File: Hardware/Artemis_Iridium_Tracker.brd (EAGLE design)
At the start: 63.5 x 69.8 mm, 199 parts, among them J1 IRIDIUM_9603N, J2 USB-C, J6 uFL, J7 SMA-, Q1 DMG3414U-7, Q2 DMG3415U-7, Q3 DMG3415U-7, Q4 2N2222, U1 CH340E_MSOP10, U10 MCP111T-240E/TT, U2 LTC3225EDDB#TRMPBF, U3 ADM4210-1, U4 UBLOX_ZOE_M8-0-10, U5 AS179-92LF, U6 MS8607-02BA01, U7 ARTEMIS_MODULESMD, U8 AP3429A, U9 MCP73831, X1 32.768kHz, X2 32.768kHz

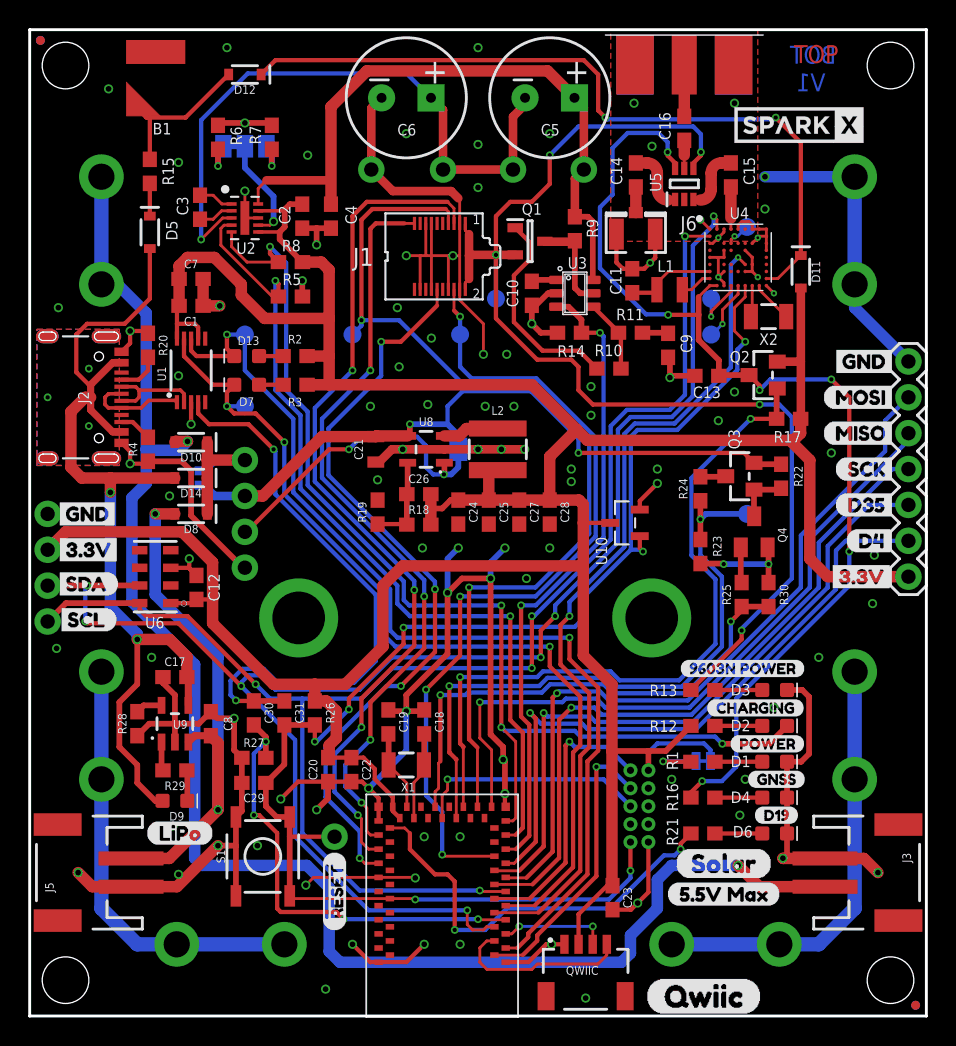
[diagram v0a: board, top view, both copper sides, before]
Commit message: Substantial update for V2 (X01) of the PCB
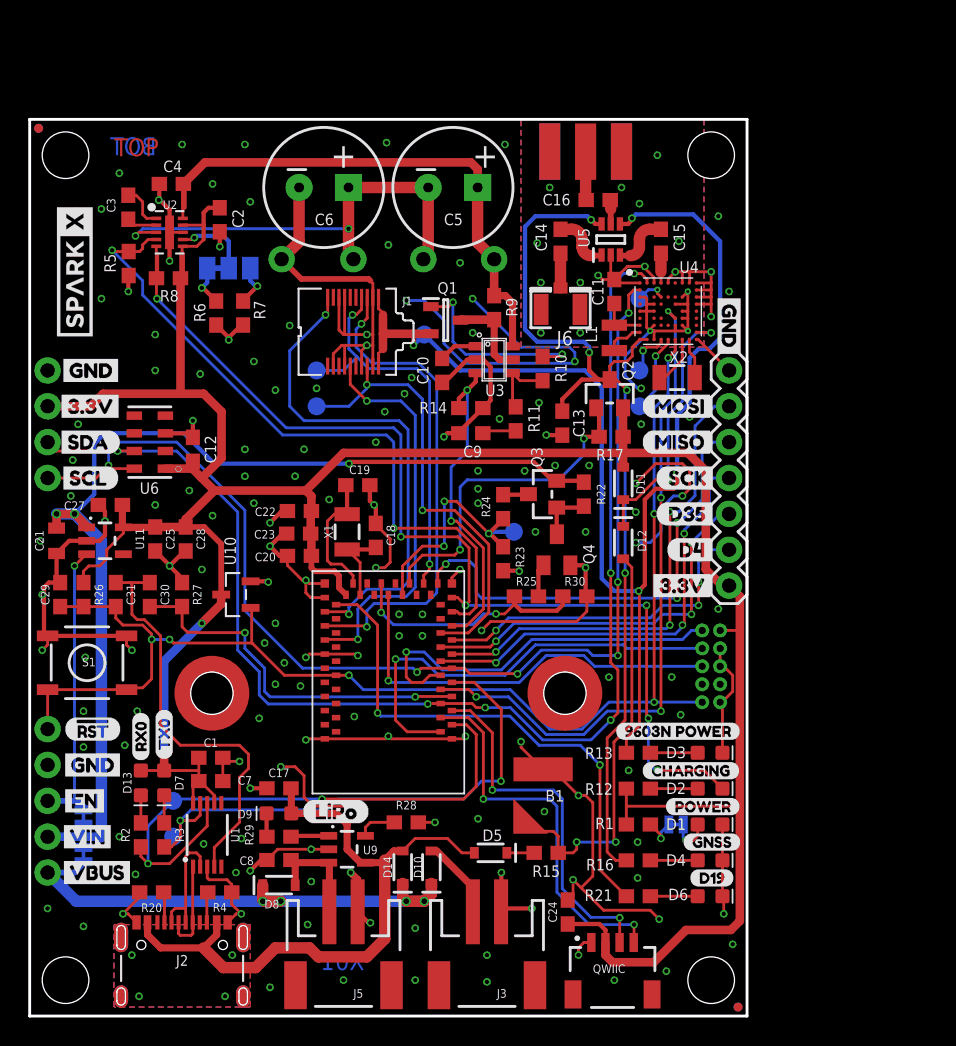
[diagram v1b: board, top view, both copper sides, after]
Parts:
- removed BAT1, BAT2, BAT3: (no value), Iridium_9603_Beacon:BATTERY-AAA-KEYSTONE82
- removed BUSV: TEST-POINT3X5, SparkFun-Connectors:PAD.03X.05
- removed C26: 22pF, SparkFun-Capacitors:0603
- removed L2: 2.2μH, SparkFun-Coils:INDUCTOR_4X4MM
- removed R18: 453k, SparkFun-Resistors:0603@2
- removed R19: 100k, SparkFun-Resistors:0603@2
- removed U$45: (no value), GND:GND0
- removed U$46: (no value), EN:EN0
- removed U$56: (no value), VBUS_3:VBUS#30
- removed U8: AP3429A, SparkFun-IC-Power:SOT23-5@1
- added U$59: (no value), GND:GND0
- added U$60: (no value), VIN:VIN0
- added U$61: (no value), 3xAA:3_X_AA0
- added U$62: (no value), 3xAAA:3_X_AAA0
- added U$63: (no value), 6VMax:6V_MAX0
- added U$64: (no value), Solar:SOLAR0
- added U$65: (no value), VINdiv3:VIN#30
- added U$66: (no value), Qwiic:QWIIC0
- added U11: 3.3V, SparkFun-IC-Power:SOT23-5
- added VIN/3: TEST-POINT3X5, SparkFun-Connectors:PAD.03X.05
- C24: value 22uF -> 1.0uF
- D10, D11, D12, D14, D8: value 3A/10V/280mV -> 0.5A/40V/420mV
- J7: value SMA- -> ANTENNA-GROUNDEDEDGE_SMA; device Qwiic_Iridium_9603N:J502-ND-142-0711-821/826_NO_CREAM -> Qwiic_Iridium_9603N:SMA-EDGE
- U$16: device RESET:#RESET0 -> TX0:TX00
- U$23: device Qwiic_Bubble:QWIIC0 -> RX0:RX00
- U$57: device Solar:SOLAR0 -> LiPo:LIPO0
- U$58: device 5V5 Max:5#5V_MAX0 -> EN:EN0
- U$7: device RESET:#RESET0 -> RST:#RST0
- moved JP9 82.6 mm to (2.54, 61.0)
- moved JP10 74.2 mm to (48.3, 61.0)
- moved JP12 66.0 mm to (48.3, 2.54)
- moved JP11 64.8 mm to (2.54, 2.54)
- moved B1 57.7 mm to (37.0, 15.6)
- moved R15 55.8 mm to (36.6, 11.6), turned to 180 degrees
- moved U$30 52.3 mm to (3.20, 52.7), turned to 90 degrees
- moved D5 50.1 mm to (32.6, 11.6), turned to 180 degrees
- moved U$58 43.6 mm to (2.03, 15.2)
- moved D12 42.6 mm to (42.0, 33.5), turned to 270 degrees
- moved U$23 39.4 mm to (7.87, 18.0), turned to 90 degrees
- moved R20 38.7 mm to (8.64, 8.76), turned to 0 degrees
- moved J2 37.6 mm to (10.8, 6.48), turned to 0 degrees
- moved 3V3EN 37.2 mm to (3.81, 14.1), turned to 90 degrees
- moved R2 35.6 mm to (7.87, 12.8), turned to 90 degrees
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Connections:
- net N$45 renamed VBUS
- removed net ARTEMIS_D0: U7.D0
- removed net ARTEMIS_D1: U7.D1
- removed net ARTEMIS_D11: U7.~AD11
- removed net ARTEMIS_D12: U7.~AD12
- removed net ARTEMIS_D14_TX1: U7.D14
- removed net ARTEMIS_D15_RX1: U7.D15
- removed net ARTEMIS_D16: U7.AD16
- removed net ARTEMIS_D2: U7.D2
- removed net ARTEMIS_D23: U7.~D23
- removed net ARTEMIS_D29: U7.~AD29
- removed net ARTEMIS_D3: U7.D3
- removed net ARTEMIS_D31: U7.~AD31
- removed net ARTEMIS_D32: U7.~AD32
- removed net ARTEMIS_D36_PDMDATA: U7.D36
- removed net ARTEMIS_D37_PDMCLK: U7.~D37
- removed net ARTEMIS_D38: U7.D38
- removed net ARTEMIS_D42: U7.~D42
- removed net ARTEMIS_D43: U7.~D43
- removed net ARTEMIS_D44: U7.~D44
- removed net ARTEMIS_D45: U7.~D45
- removed net N$33: L2.P$1, U8.3
- removed net N$34: D13.A, R2.1
- removed net N$38: BAT1.GND@1, BAT1.GND@2, BAT2.PWR@1, BAT2.PWR@2
- removed net N$42: BAT1.PWR@1, BAT1.PWR@2, D10.A, J3.2
- removed net N$43: BAT2.GND@1, BAT2.GND@2, BAT3.PWR@1, BAT3.PWR@2
- new net V_AAA: D10.A, J3.2
- net 3.3V: now also D13.A, D7.A, R1.2, U11.5; no longer C26.1, JP2.2, L2.P$2, R18.2, R2.2, R3.2
- net ANTENNA: now also J7.SIG; no longer J7.1
- net ARTEMIS_D13: now also VIN/3.P$1; no longer BUSV.P$1
- net ARTEMIS_RX0: now also R2.1; no longer D13.C
- net ARTEMIS_TX0: now also R3.1; no longer D7.C
- net GND: now also J7.GND@0, J7.GND@1, J7.GND@2, J7.GND@3, U11.2; no longer BAT3.GND@1, BAT3.GND@2, J7.G@1, J7.G@2, J7.G@3, J7.G@4, R19.1, U8.2
- net N$22: now also D13.C, R2.2; no longer D7.A, R3.1
- net N$23: now also JP2.1; no longer R1.1
- net N$3: now also JP2.2, R1.1; no longer JP2.1, R1.2
- net N$32: now also D7.C, R3.2; no longer C26.2, R18.1, R19.2, U8.5
- net N$36: now also U11.3; no longer U8.1
- net VIN: now also U11.1; no longer U8.4
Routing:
- net N$42: track 112.4 -> 0.00 mm, vias 2 -> 0
- net 3.3V: track 247.8 -> 196.1 mm, vias 0 -> 2
- net ARTEMIS_D25: track 67.9 -> 28.6 mm
- net N$24: track 53.8 -> 19.0 mm
- net V_BATT: track 39.0 -> 8.15 mm, vias 2 -> 0
- net N$43: track 30.8 -> 0.00 mm
- net N$38: track 30.8 -> 0.00 mm
- net ARTEMIS_RX0: track 71.2 -> 41.1 mm
- net ARTEMIS_D13: track 46.4 -> 17.5 mm, vias 2 -> 3
- net ARTEMIS_D26: track 51.3 -> 23.8 mm
- net VBUS: track 11.0 -> 38.0 mm, vias 0 -> 4
- net ARTEMIS_D24: track 59.2 -> 32.4 mm, vias 4 -> 2
- net ARTEMIS_D17: track 61.8 -> 35.2 mm, vias 4 -> 2
- net VIN: track 49.7 -> 76.0 mm, vias 2 -> 3
- net ARTEMIS_D41: track 53.7 -> 28.2 mm, vias 4 -> 2
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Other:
- board size 63.5 x 69.8 mm -> 50.8 x 63.5 mm
- board text added: "X01"
- board text removed: "V1"
